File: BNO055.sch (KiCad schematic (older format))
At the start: 13 parts, among them SW2 SW_Push, U4 BNO055, Y2 32.768kHz

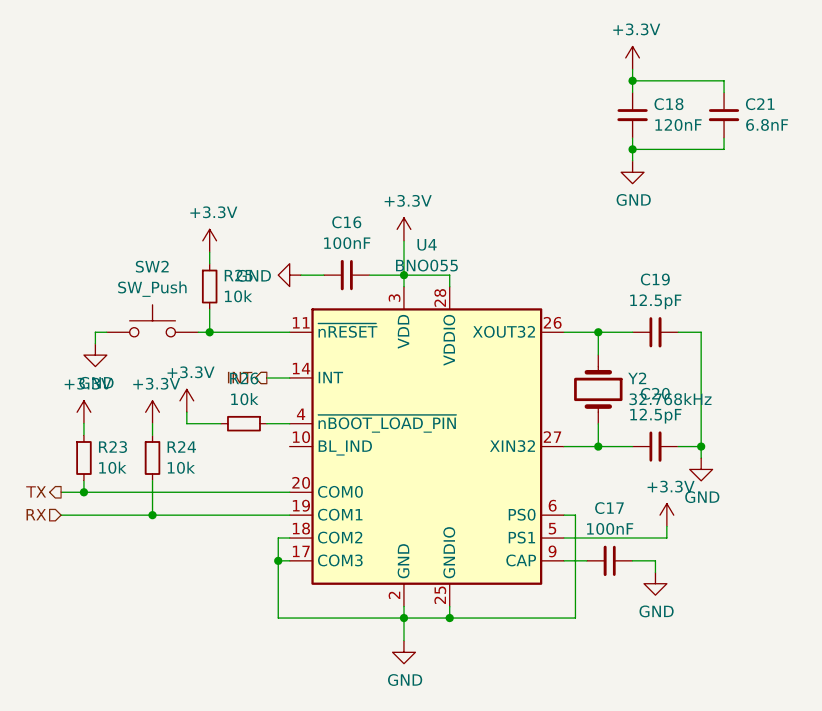
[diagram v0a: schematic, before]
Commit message: layout
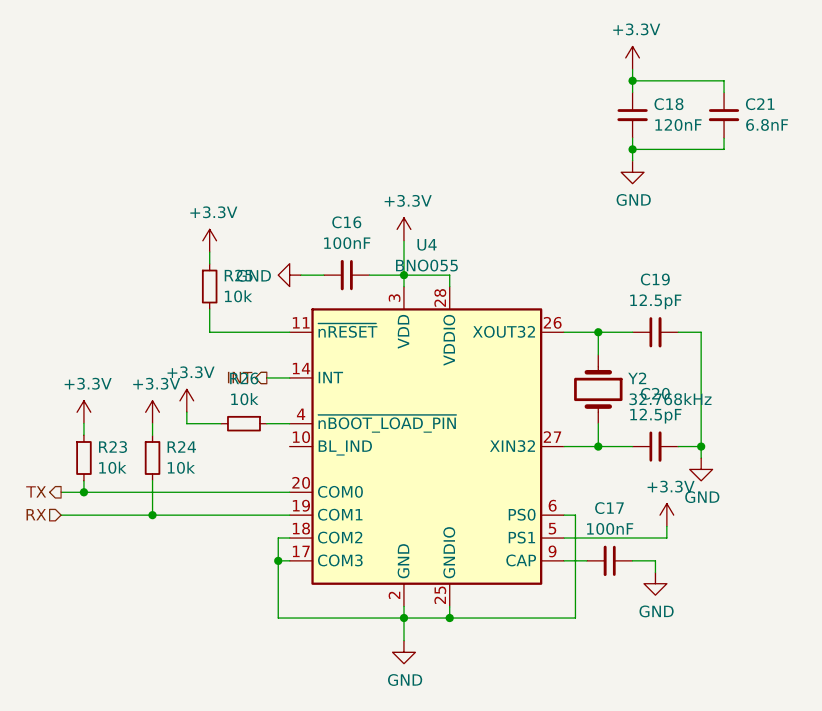
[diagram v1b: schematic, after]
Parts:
- removed SW2: SW_Push, Button_Switch_SMD:SW_SPST_PTS810, symbol Switch:SW_Push
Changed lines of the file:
@@
 $EndComp
-$Comp
-L Switch:SW_Push SW?
-U 1 1 5C994ABC
-P 4850 2750
-AR Path="/5C8FB8FD/5C994ABC" Ref="SW?"  Part="1"
-AR Path="/5C9128F0/5C994ABC" Ref="SW2"  Part="1"
-F 0 "SW2" H 4850 3035 50  0000 C CNN
-F 1 "SW_Push" H 4850 2944 50  0000 C CNN
-F 2 "Button_Switch_SMD:SW_SPST_PTS810" H 4850 2950 50  0001 C CNN
-F 3 "~" H 4850 2950 50  0001 C CNN
-	1    4850 2750
-	1    0    0    -1
-$EndComp
-Wire Wire Line
-	4650 2750 4600 2750
-Wire Wire Line
-	4600 2750 4600 2800
-$Comp
-L power:GND #PWR?
-U 1 1 5C994AC5
-P 4600 2800
-AR Path="/5C8FB8FD/5C994AC5" Ref="#PWR?"  Part="1"
-AR Path="/5C9128F0/5C994AC5" Ref="#PWR043"  Part="1"
-F 0 "#PWR043" H 4600 2550 50  0001 C CNN
-F 1 "GND" H 4605 2627 50  0000 C CNN
-F 2 "" H 4600 2800 50  0001 C CNN
-F 3 "" H 4600 2800 50  0001 C CNN
-	1    4600 2800
-	1    0    0    -1
-$EndComp
-Wire Wire Line
-	5050 2750 5100 2750
 $Comp
 L Device:R_Small R25
@@
 Wire Wire Line
 	5100 2650 5100 2750
-Connection ~ 5100 2750
 Wire Wire Line
 	5100 2750 5450 2750
